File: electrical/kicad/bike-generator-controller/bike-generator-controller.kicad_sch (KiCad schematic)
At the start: 0 parts

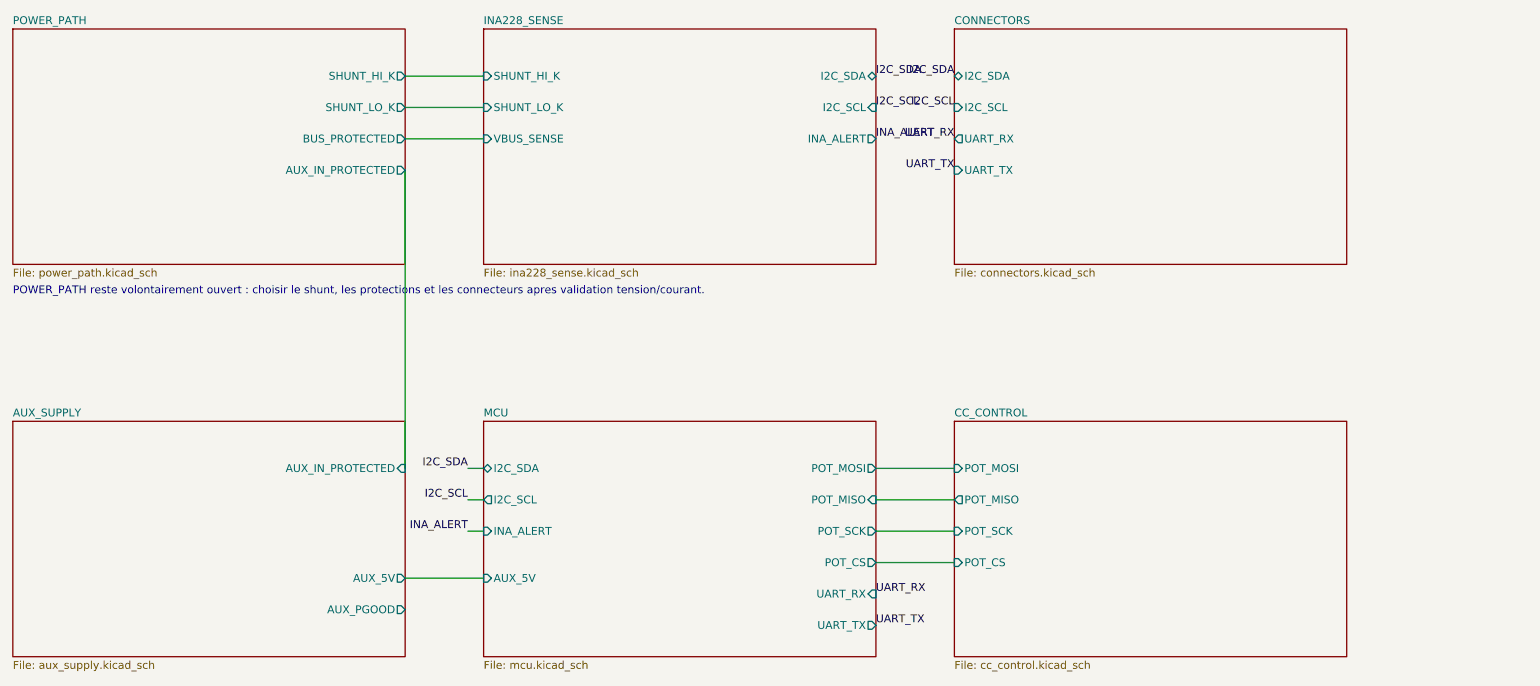
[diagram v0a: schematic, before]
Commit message: feat: establish controller PCB V1 design baseline
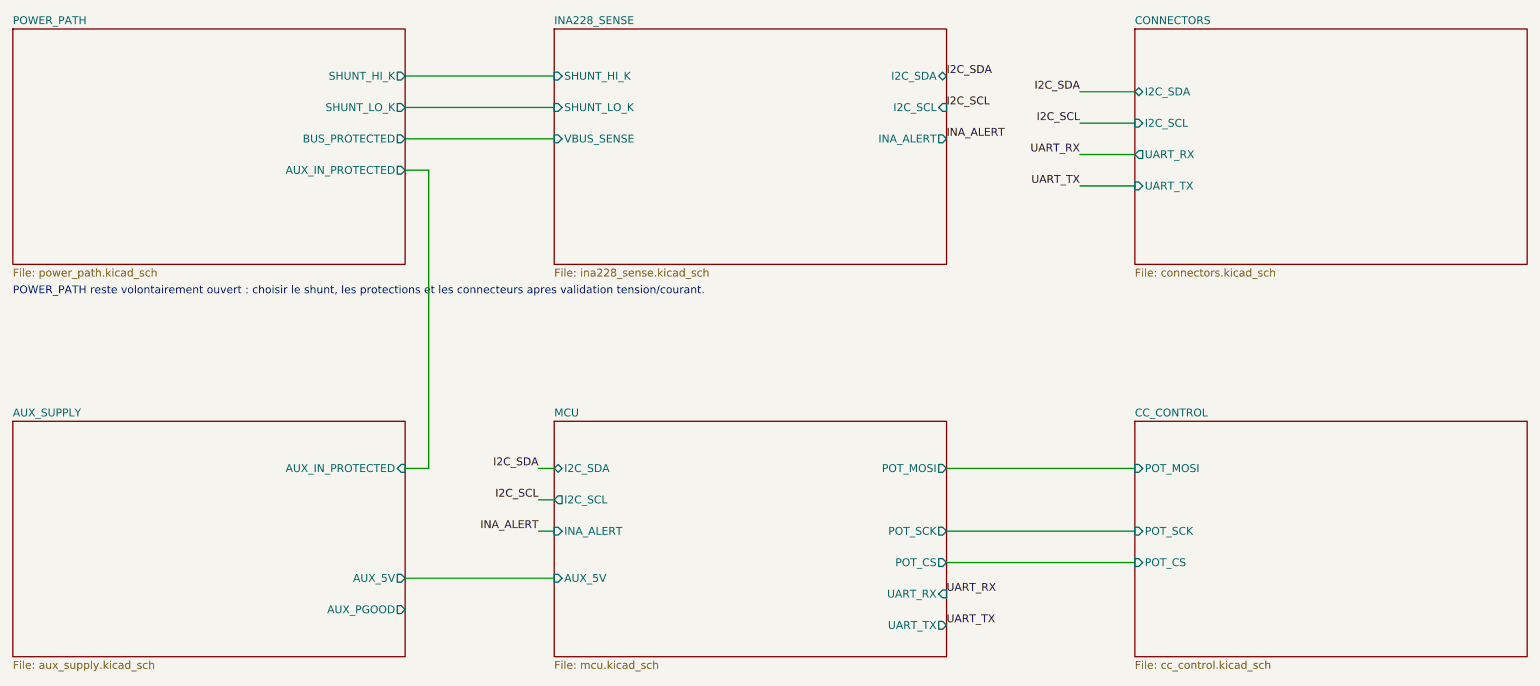
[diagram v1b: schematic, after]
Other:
- sheet CC_CONTROL ports: added none; removed POT_MISO
- sheet MCU ports: added none; removed POT_MISO
